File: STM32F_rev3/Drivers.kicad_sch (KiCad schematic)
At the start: 28 parts, among them Q1 ISL9V5045S3ST, Q2 ISL9V5045S3ST, Q3 ISL9V5045S3ST, Q4 ISL9V5045S3ST

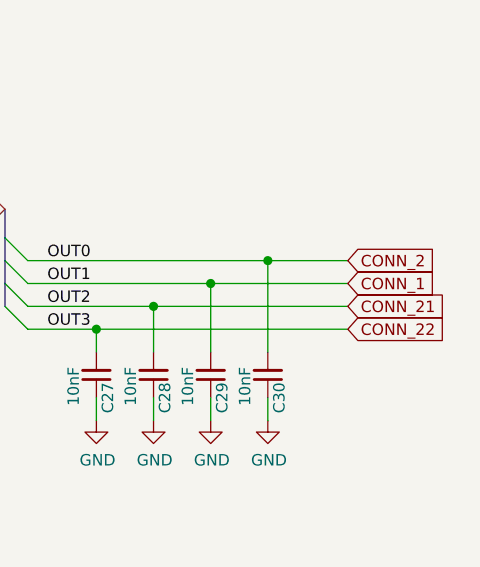
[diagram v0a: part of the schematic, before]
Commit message: Update on PMIC
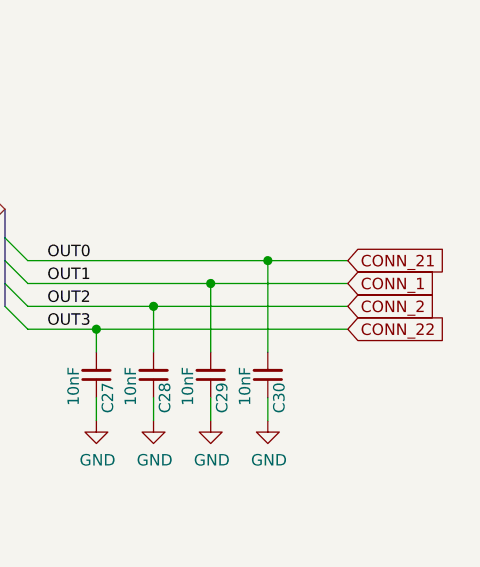
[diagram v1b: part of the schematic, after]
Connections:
- net CONN_2: now also C28.2; no longer C30.2
- net CONN_21: now also C30.2; no longer C28.2
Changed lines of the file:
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@@
 (kicad_sch (version 20201015) (generator eeschema)
-  (page 1 5)
+  (page 1 6)
   (paper "A4")
   (junction (at 49.53 170.18) (diameter 1.016) (color 0 0 0 0))
@@
     (effects (font (size 1.27 1.27)) (justify left))
   )
-  (global_label "CONN_2" (shape input) (at 165.1 147.32 0)
+  (global_label "CONN_21" (shape input) (at 165.1 147.32 0)
     (effects (font (size 1.27 1.27)) (justify left))
   )
@@
     (effects (font (size 1.27 1.27)) (justify left))
   )
-  (global_label "CONN_21" (shape input) (at 165.1 152.4 0)
-    (effects (font (size 1.27 1.27)) (justify left))
-  )
+  (global_label "CONN_2" (shape input) (at 165.1 152.4 0)
+    (effects (font (size 1.27 1.27)) (justify left))
+  )

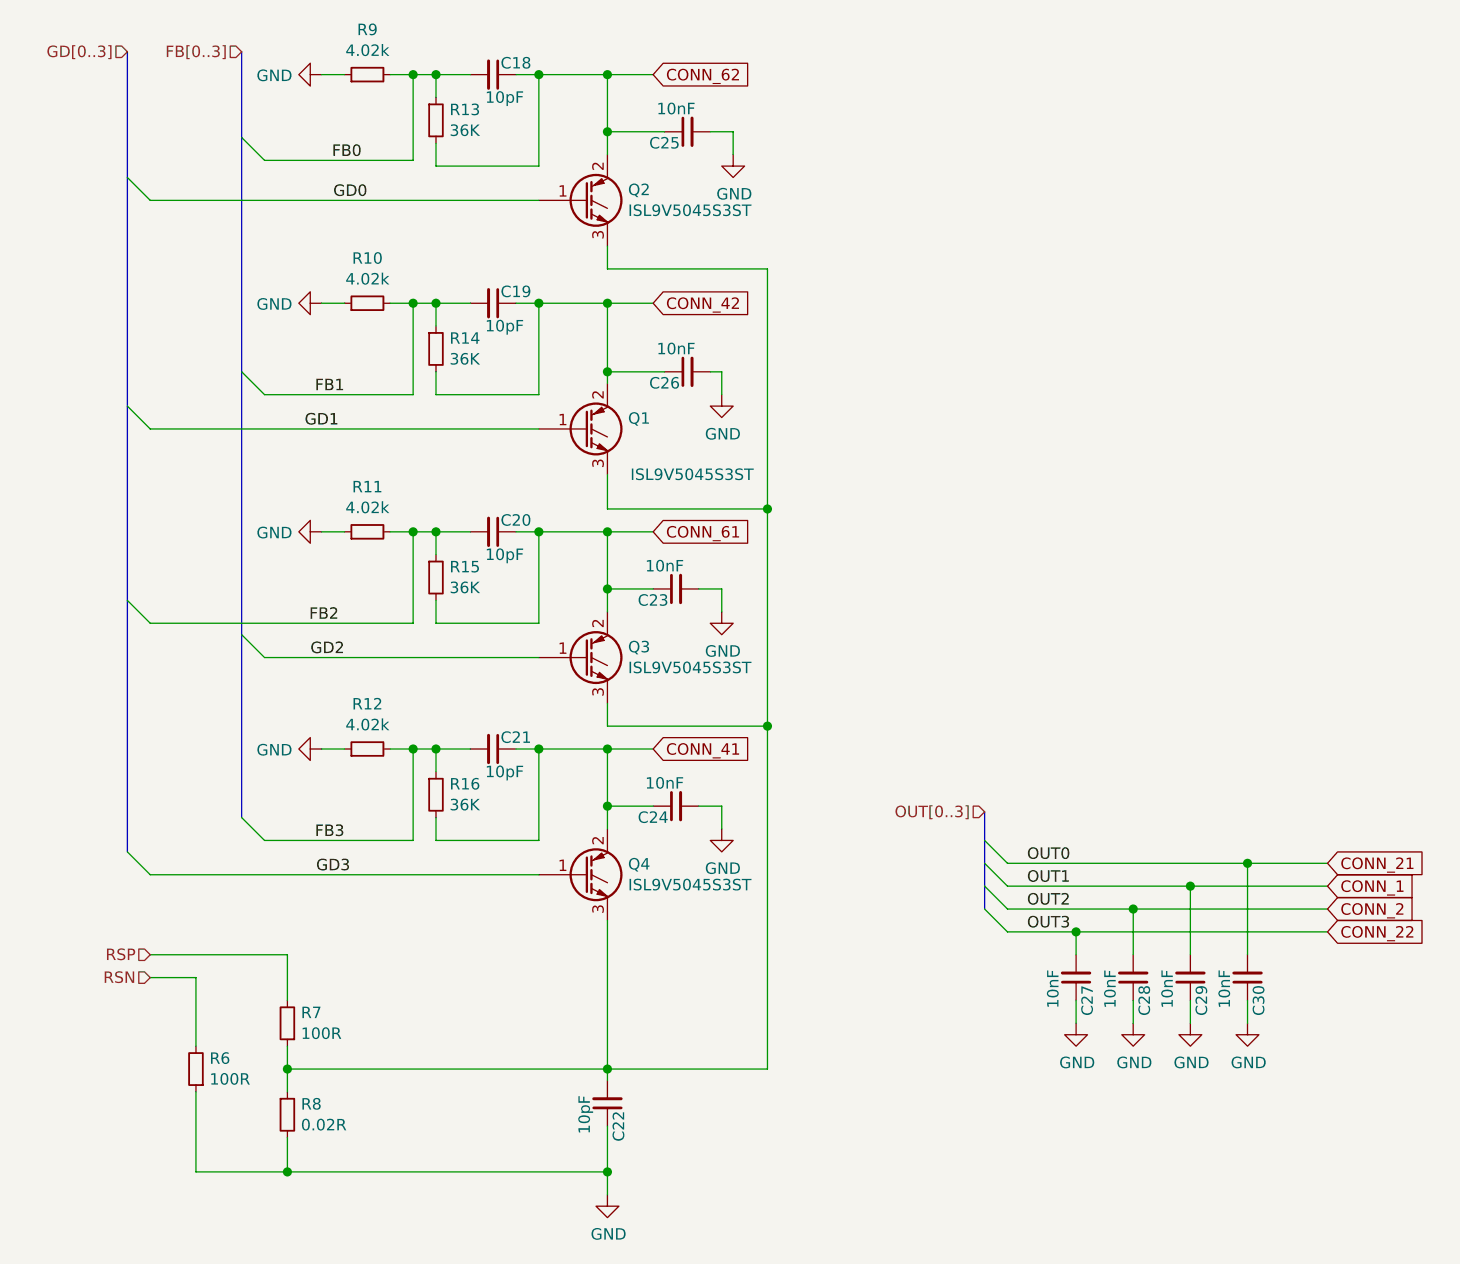
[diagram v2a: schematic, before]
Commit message: Last commit to rev3
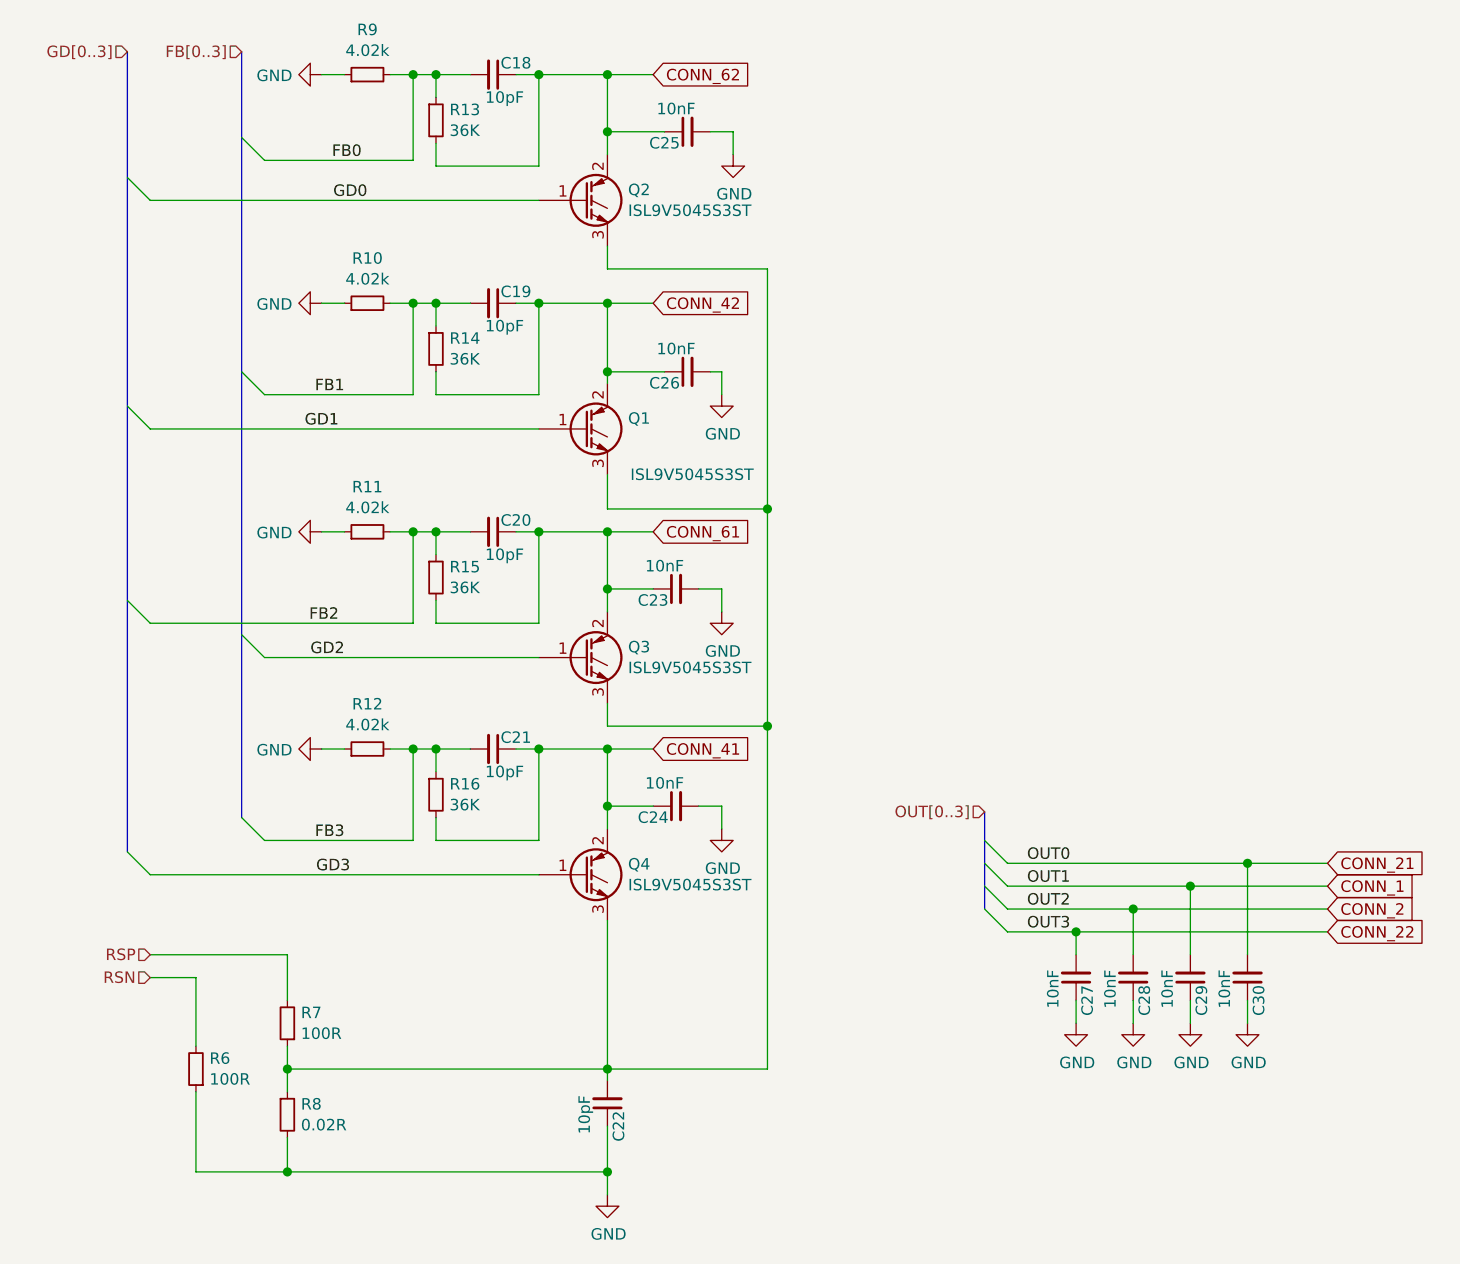
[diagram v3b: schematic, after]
